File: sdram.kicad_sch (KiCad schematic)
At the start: 25 parts, among them U1 MT48LC16M16A2P, U8 T8Q144xx, X2 ECS-2520MV-120-CM

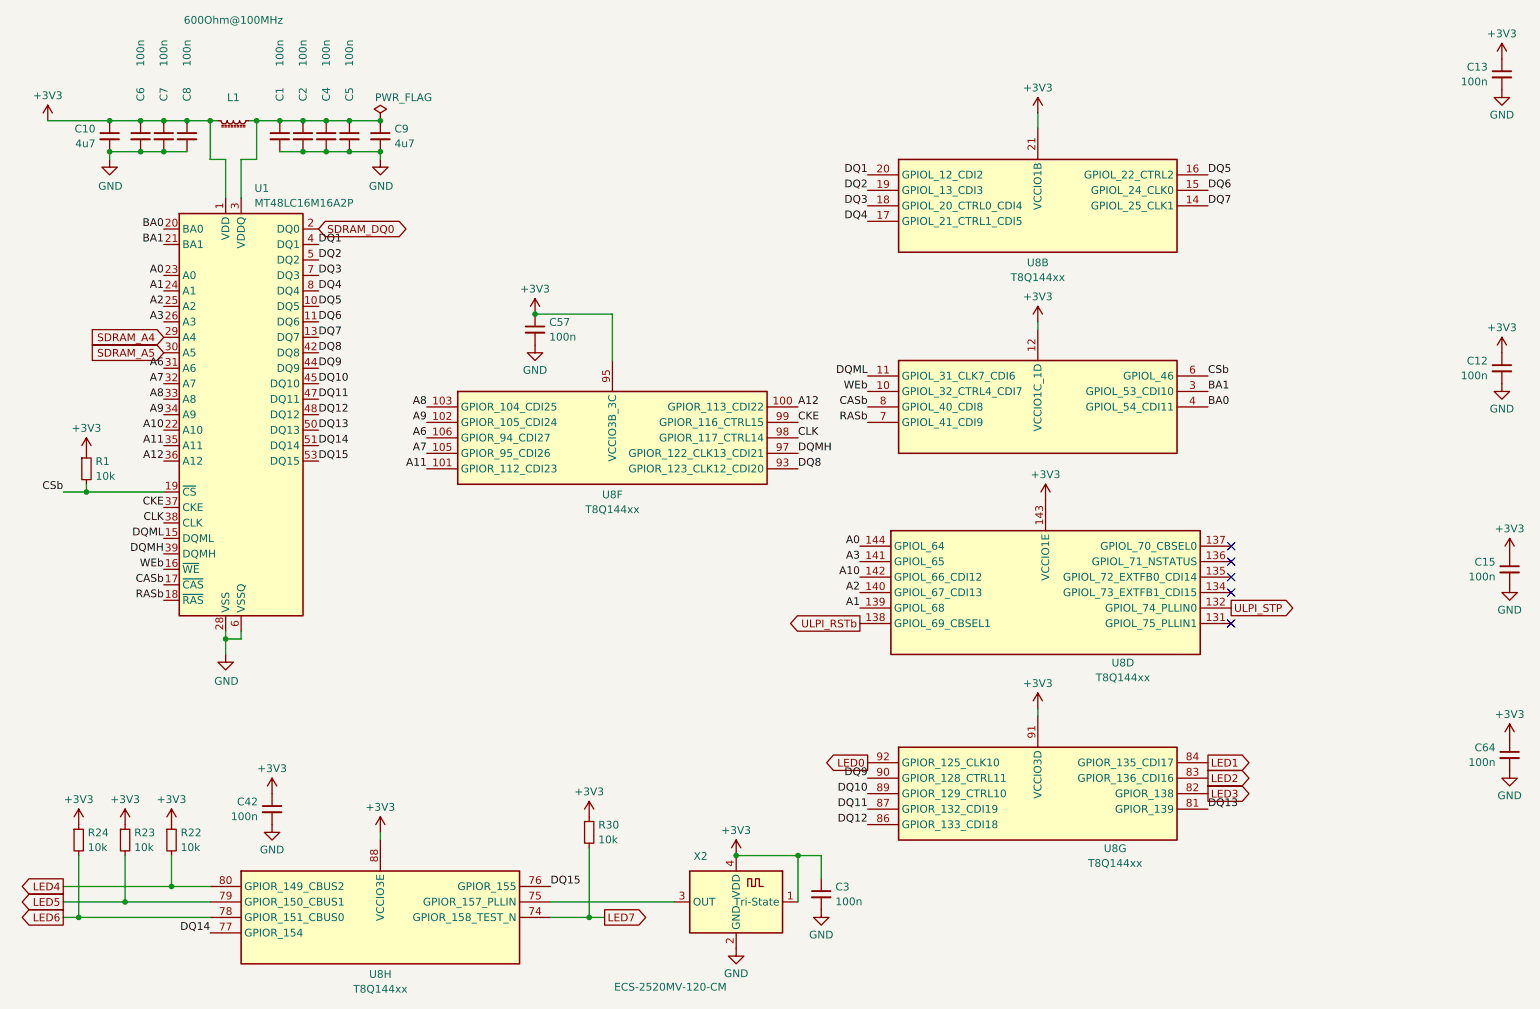
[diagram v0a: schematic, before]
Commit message: added ethernet phy
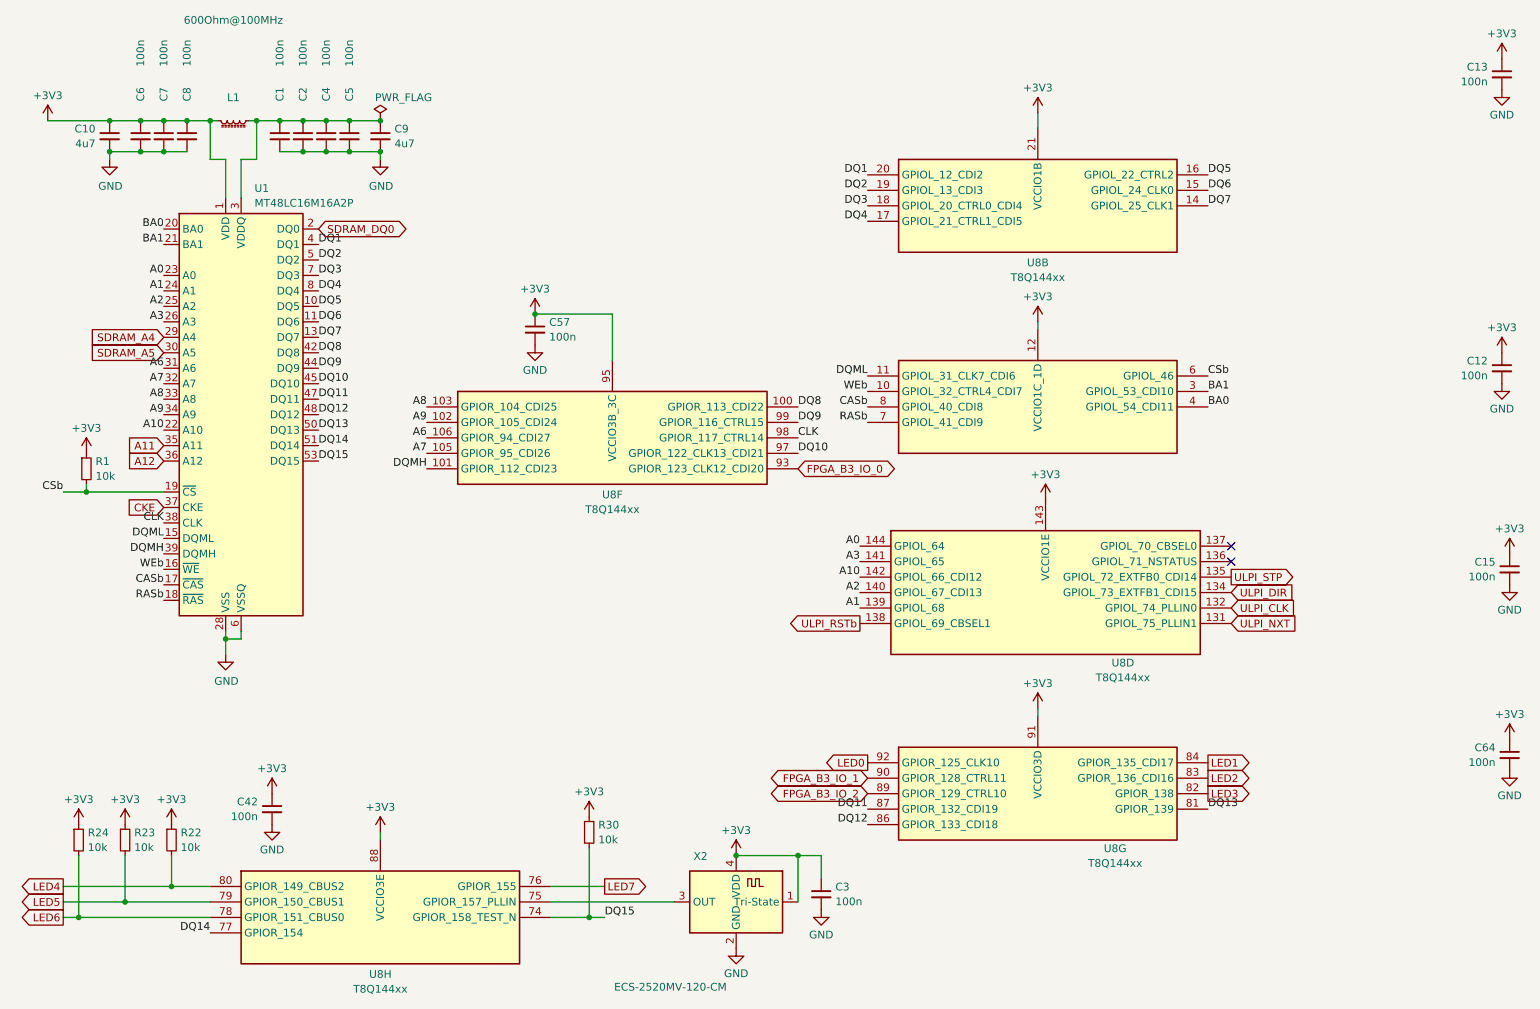
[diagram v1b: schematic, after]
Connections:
- net A11: no longer U8.101 (GPIOR_112_CDI23)
- net A12: no longer U8.100 (GPIOR_113_CDI22)
- net CKE: no longer U8.99 (GPIOR_116_CTRL15)
- net DQ10: now also U8.97 (GPIOR_122_CLK13_CDI21); no longer U8.89 (GPIOR_129_CTRL10)
- net DQ15: now also R30.2, U8.74 (GPIOR_158_TEST_N); no longer U8.76 (GPIOR_155)
- net DQ8: now also U8.100 (GPIOR_113_CDI22); no longer U8.93 (GPIOR_123_CLK12_CDI20)
- net DQ9: now also U8.99 (GPIOR_116_CTRL15); no longer U8.90 (GPIOR_128_CTRL11)
- net DQMH: now also U8.101 (GPIOR_112_CDI23); no longer U8.97 (GPIOR_122_CLK13_CDI21)
- net LED7: now also U8.76 (GPIOR_155); no longer R30.2, U8.74 (GPIOR_158_TEST_N)
- net ULPI_STP: now also U8.135 (GPIOL_72_EXTFB0_CDI14); no longer U8.132 (GPIOL_74_PLLIN0)
- net ULPI_NXT: now reaches U8.131 (GPIOL_75_PLLIN1)
- net ULPI_DIR: now reaches U8.134 (GPIOL_73_EXTFB1_CDI15)
- new net FPGA_B3_IO_0: U8.93 (GPIOR_123_CLK12_CDI20)
- new net FPGA_B3_IO_1: U8.90 (GPIOR_128_CTRL11)
- new net FPGA_B3_IO_2: U8.89 (GPIOR_129_CTRL10)
- new net ULPI_CLK: U8.132 (GPIOL_74_PLLIN0)
- no-connect marks 5 -> 2
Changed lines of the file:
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@@
   (junction (at 74.93 40.64) (diameter 0) (color 0 0 0 0)
   )
-  (no_connect (at 219.71 123.19))
   (no_connect (at 219.71 113.03))
-  (no_connect (at 219.71 115.57))
-  (no_connect (at 219.71 118.11))
   (no_connect (at 219.71 110.49))
   (wire (pts (xy 107.95 168.91) (xy 128.27 168.91))
@@
     (stroke (width 0) (type default))
   )
+  (wire (pts (xy 116.84 166.37) (xy 107.95 166.37))
+    (stroke (width 0) (type default))
+  )
   (wire (pts (xy 74.93 40.64) (xy 80.01 40.64))
     (stroke (width 0) (type default))
@@
     (effects (font (size 1.27 1.27)) (justify right bottom))
   )
-  (label "CKE" (at 148.59 90.17 0) (fields_autoplaced)
-    (effects (font (size 1.27 1.27)) (justify left bottom))
-  )
   (label "DQ11" (at 160.02 153.67 180) (fields_autoplaced)
     (effects (font (size 1.27 1.27)) (justify right bottom))
@@
     (effects (font (size 1.27 1.27)) (justify right bottom))
   )
-  (label "A11" (at 44.45 93.98 180) (fields_autoplaced)
-    (effects (font (size 1.27 1.27)) (justify right bottom))
-  )
   (label "DQMH" (at 44.45 111.76 180) (fields_autoplaced)
     (effects (font (size 1.27 1.27)) (justify right bottom))
   )
-  (label "DQ10" (at 160.02 151.13 180) (fields_autoplaced)
-    (effects (font (size 1.27 1.27)) (justify right bottom))
+  (label "DQ10" (at 148.59 95.25 0) (fields_autoplaced)
+    (effects (font (size 1.27 1.27)) (justify left bottom))
   )
   (label "DQ13" (at 215.9 153.67 0) (fields_autoplaced)
     (effects (font (size 1.27 1.27)) (justify left bottom))
   )
-  (label "DQ9" (at 160.02 148.59 180) (fields_autoplaced)
-    (effects (font (size 1.27 1.27)) (justify right bottom))
-  )
-  (label "CKE" (at 44.45 104.14 180) (fields_autoplaced)
-    (effects (font (size 1.27 1.27)) (justify right bottom))
+  (label "DQ9" (at 148.59 90.17 0) (fields_autoplaced)
+    (effects (font (size 1.27 1.27)) (justify left bottom))
   )
   (label "DQ4" (at 69.85 68.58 0) (fields_autoplaced)
@@
     (effects (font (size 1.27 1.27)) (justify right bottom))
   )
-  (label "A11" (at 87.63 97.79 180) (fields_autoplaced)
-    (effects (font (size 1.27 1.27)) (justify right bottom))
-  )
   (label "A3" (at 158.75 113.03 180) (fields_autoplaced)
     (effects (font (size 1.27 1.27)) (justify right bottom))
@@
     (effects (font (size 1.27 1.27)) (justify left bottom))
   )
-  (label "DQ15" (at 107.95 166.37 0) (fields_autoplaced)
+  (label "DQ15" (at 116.84 171.45 0) (fields_autoplaced)
     (effects (font (size 1.27 1.27)) (justify left bottom))
   )
@@
     (effects (font (size 1.27 1.27)) (justify right bottom))
   )
-  (label "A12" (at 148.59 87.63 0) (fields_autoplaced)
-    (effects (font (size 1.27 1.27)) (justify left bottom))
-  )
   (label "DQ7" (at 215.9 54.61 0) (fields_autoplaced)
     (effects (font (size 1.27 1.27)) (justify left bottom))
   )
-  (label "DQ8" (at 148.59 97.79 0) (fields_autoplaced)
+  (label "DQ8" (at 148.59 87.63 0) (fields_autoplaced)
     (effects (font (size 1.27 1.27)) (justify left bottom))
   )
@@
     (effects (font (size 1.27 1.27)) (justify left bottom))
   )
-  (label "A12" (at 44.45 96.52 180) (fields_autoplaced)
-    (effects (font (size 1.27 1.27)) (justify right bottom))
-  )
   (label "A6" (at 44.45 81.28 180) (fields_autoplaced)
     (effects (font (size 1.27 1.27)) (justify right bottom))
   )
-  (label "DQMH" (at 148.59 95.25 0) (fields_autoplaced)
-    (effects (font (size 1.27 1.27)) (justify left bottom))
+  (label "DQMH" (at 87.63 97.79 180) (fields_autoplaced)
+    (effects (font (size 1.27 1.27)) (justify right bottom))
   )
   (label "DQ14" (at 69.85 93.98 0) (fields_autoplaced)
@@
     )
   )
-  (global_label "LED7" (shape output) (at 116.84 171.45 0) (fields_autoplaced)
-    (effects (font (size 1.27 1.27)) (justify left))
-    (property "Intersheetrefs" "${INTERSHEET_REFS}" (at 124.4818 171.45 0)
+  (global_label "ULPI_NXT" (shape input) (at 219.71 123.19 0) (fields_autoplaced)
+    (effects (font (size 1.27 1.27)) (justify left))
+    (property "Intersheetrefs" "${INTERSHEET_REFS}" (at 231.4038 123.19 0)
+      (effects (font (size 1.27 1.27)) (justify left) hide)
+    )
+  )
+  (global_label "FPGA_B3_IO_0" (shape bidirectional) (at 148.59 97.79 0) (fields_autoplaced)
+    (effects (font (size 1.27 1.27)) (justify left))
+    (property "Intersheetrefs" "${INTERSHEET_REFS}" (at 165.9308 97.79 0)
+      (effects (font (size 1.27 1.27)) (justify left) hide)
+    )
+  )
+  (global_label "LED7" (shape output) (at 116.84 166.37 0) (fields_autoplaced)
+    (effects (font (size 1.27 1.27)) (justify left))
+    (property "Intersheetrefs" "${INTERSHEET_REFS}" (at 124.4818 166.37 0)
       (effects (font (size 1.27 1.27)) (justify left) hide)
     )
@@
     )
   )
+  (global_label "ULPI_CLK" (shape input) (at 219.71 120.65 0) (fields_autoplaced)
+    (effects (font (size 1.27 1.27)) (justify left))
+    (property "Intersheetrefs" "${INTERSHEET_REFS}" (at 231.4643 120.65 0)
+      (effects (font (size 1.27 1.27)) (justify left) hide)
+    )
+  )
   (global_label "LED2" (shape output) (at 215.9 148.59 0) (fields_autoplaced)
     (effects (font (size 1.27 1.27)) (justify left))
@@
     )
   )
+  (global_label "FPGA_B3_IO_1" (shape bidirectional) (at 160.02 148.59 180) (fields_autoplaced)
+    (effects (font (size 1.27 1.27)) (justify right))
+    (property "Intersheetrefs" "${INTERSHEET_REFS}" (at 142.6792 148.59 0)
+      (effects (font (size 1.27 1.27)) (justify right) hide)
+    )
+  )
+  (global_label "FPGA_B3_IO_2" (shape bidirectional) (at 160.02 151.13 180) (fields_autoplaced)
+    (effects (font (size 1.27 1.27)) (justify right))
+    (property "Intersheetrefs" "${INTERSHEET_REFS}" (at 142.6792 151.13 0)
+      (effects (font (size 1.27 1.27)) (justify right) hide)
+    )
+  )
+  (global_label "A12" (shape input) (at 44.45 96.52 180) (fields_autoplaced)
+    (effects (font (size 1.27 1.27)) (justify right))
+    (property "Intersheetrefs" "${INTERSHEET_REFS}" (at 37.9572 96.52 0)
+      (effects (font (size 1.27 1.27)) (justify right) hide)
+    )
+  )
   (global_label "LED1" (shape output) (at 215.9 146.05 0) (fields_autoplaced)
     (effects (font (size 1.27 1.27)) (justify left))
@@
     )
   )
-  (global_label "ULPI_STP" (shape output) (at 219.71 120.65 0) (fields_autoplaced)
-    (effects (font (size 1.27 1.27)) (justify left))
-    (property "Intersheetrefs" "${INTERSHEET_REFS}" (at 231.3433 120.65 0)
+  (global_label "ULPI_STP" (shape output) (at 219.71 115.57 0) (fields_autoplaced)
+    (effects (font (size 1.27 1.27)) (justify left))
+    (property "Intersheetrefs" "${INTERSHEET_REFS}" (at 231.3433 115.57 0)
       (effects (font (size 1.27 1.27)) (justify left) hide)
     )
@@
       (effects (font (size 1.27 1.27)) (justify right) hide)
     )
+  )
+  (global_label "CKE" (shape input) (at 44.45 104.14 180) (fields_autoplaced)
+    (effects (font (size 1.27 1.27)) (justify right))
+    (property "Intersheetrefs" "${INTERSHEET_REFS}" (at 37.7758 104.14 0)
+      (effects (font (size 1.27 1.27)) (justify right) hide)
+    )
+  )
+  (global_label "ULPI_DIR" (shape input) (at 219.71 118.11 0) (fields_autoplaced)
+    (effects (font (size 1.27 1.27)) (justify left))
+    (property "Intersheetrefs" "${INTERSHEET_REFS}" (at 231.041 118.11 0)
+      (effects (font (size 1.27 1.27)) (justify left) hide)
+    )
+  )
+  (global_label "A11" (shape input) (at 44.45 93.98 180) (fields_autoplaced)
+    (effects (font (size 1.27 1.27)) (justify right))
+    (property "Intersheetrefs" "${INTERSHEET_REFS}" (at 37.9572 93.98 0)
+      (effects (font (size 1.27 1.27)) (justify right) hide)
+    )
